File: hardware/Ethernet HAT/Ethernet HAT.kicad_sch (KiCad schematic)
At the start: 3 parts, among them J1 RJ45_Amphenol_RJMG1BD3B8K1ANR, J2 Conn_01x10_Pin, U1 W5500

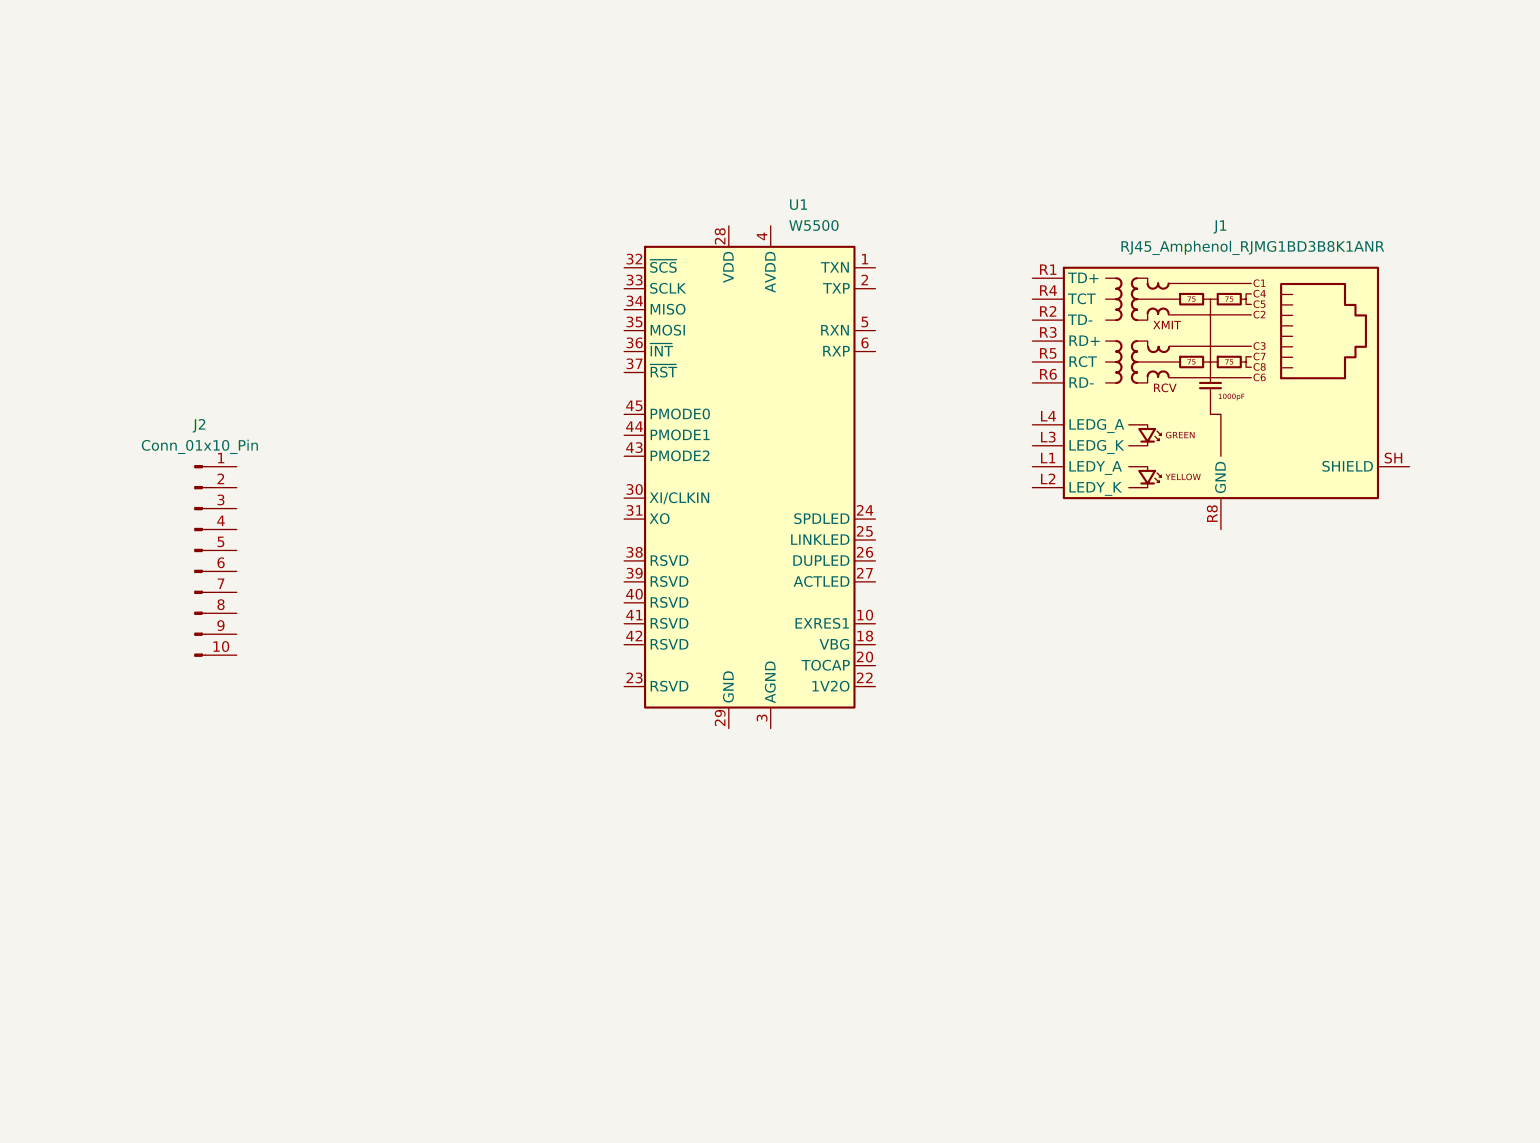
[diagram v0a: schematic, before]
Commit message: EthernetHat ordered
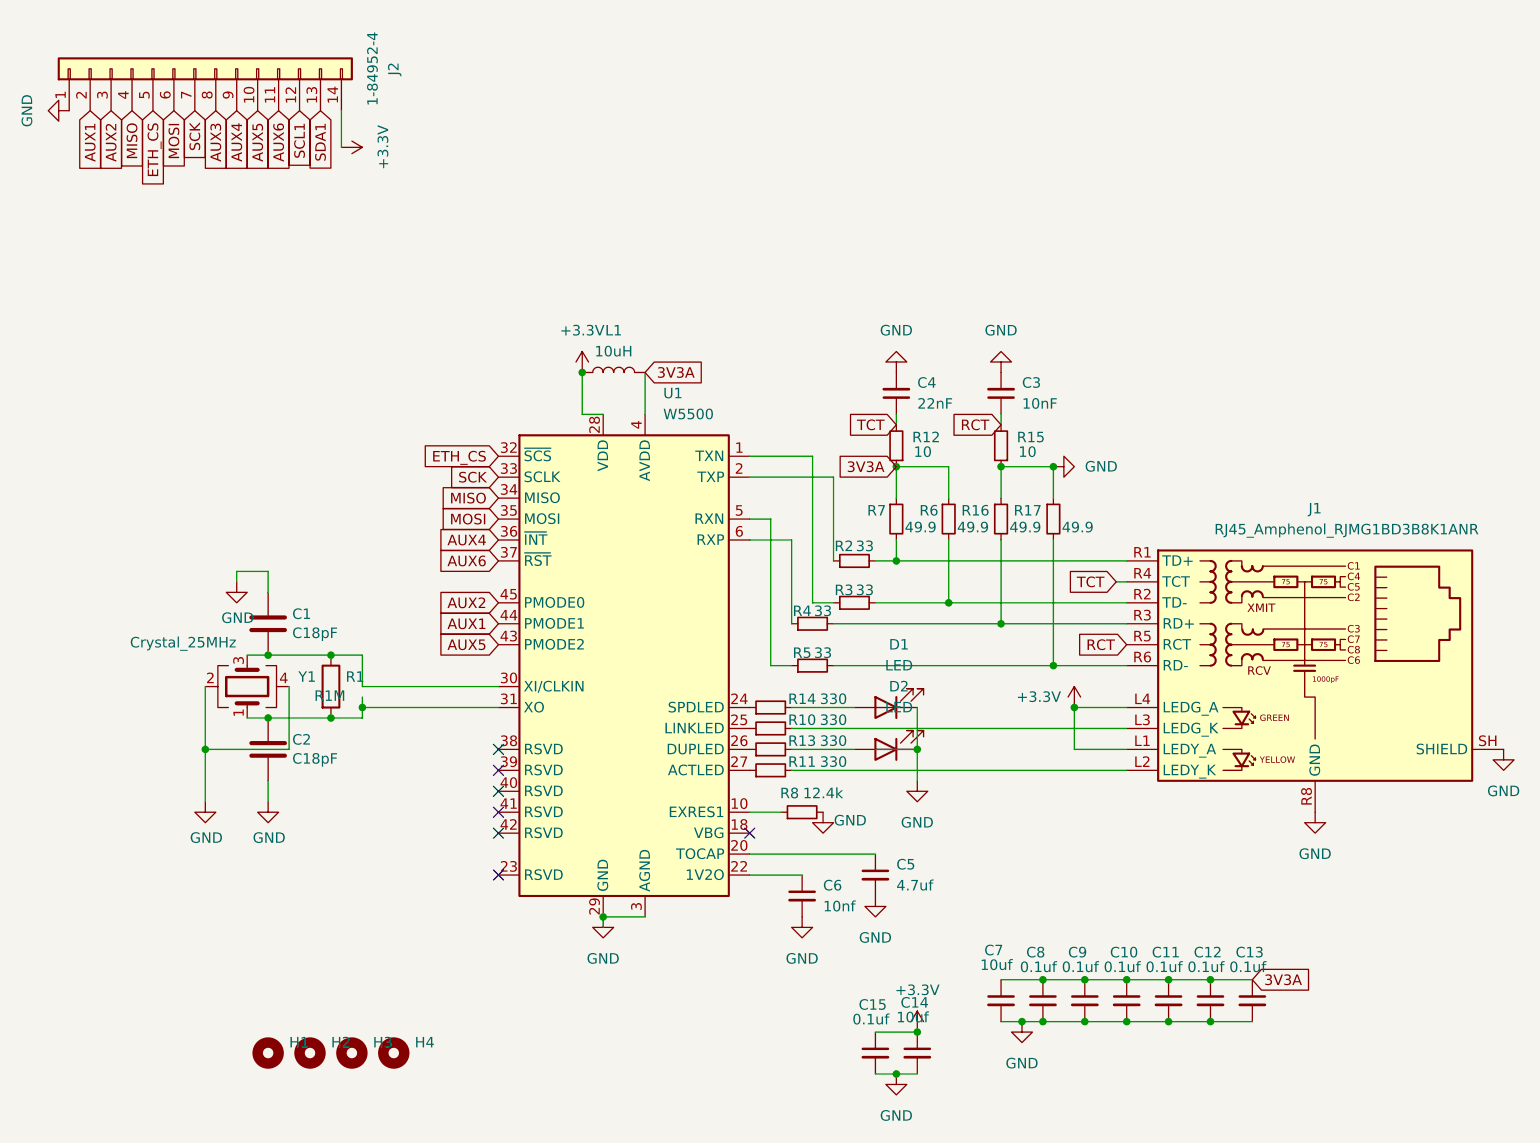
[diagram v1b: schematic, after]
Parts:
- removed J2: Conn_01x10_Pin, Connector_PinHeader_2.54mm:PinHeader_2x05_P2.54mm_Vertical, symbol Connector:Conn_01x10_Pin
- added C1, C2: C18pF, Capacitor_SMD:C_0402_1005Metric, symbol Device:C
- added C10, C11, C12, C13, C15, C8, C9: 0.1uf, Capacitor_SMD:C_0402_1005Metric, symbol Device:C_Small
- added C14, C7: 10uf, Capacitor_SMD:C_0805_2012Metric, symbol Device:C_Small
- added C3: 10nF, Capacitor_SMD:C_0402_1005Metric, symbol Device:C_Small
- added C4: 22nF, Capacitor_SMD:C_0402_1005Metric, symbol Device:C_Small
- added C5: 4.7uf, Capacitor_SMD:C_0402_1005Metric, symbol Device:C_Small
- added C6: 10nf, Capacitor_SMD:C_0402_1005Metric, symbol Device:C_Small
- added D1, D2: LED, LED_SMD:LED_0603_1608Metric, symbol Device:LED
- added H1, H2, H3, H4: MountingHole, MountingHole:MountingHole_3.2mm_M3_ISO14580_Pad, symbol Mechanical:MountingHole
- added J2: 1-84952-4, Connector_FFC-FPC:TE_1-84952-4_1x14-1MP_P1.0mm_Horizontal, symbol Connector_Generic:Conn_01x14
- added L1: 10uH, Inductor_SMD:L_0603_1608Metric, symbol Device:L
- added R1: R1M, Resistor_SMD:R_0402_1005Metric, symbol Device:R
- added R10, R11, R13, R14: 330, Resistor_SMD:R_0402_1005Metric, symbol Device:R_Small
- added R12, R15: 10, Resistor_SMD:R_0402_1005Metric, symbol Device:R_Small
- added R16, R17, R6, R7: 49.9, Resistor_SMD:R_0402_1005Metric, symbol Device:R_Small
- added R2, R3, R4, R5: 33, Resistor_SMD:R_0402_1005Metric, symbol Device:R_Small
- added R8: 12.4k, Resistor_SMD:R_0402_1005Metric, symbol Device:R_Small
- added Y1: Crystal_25MHz, Crystal:Crystal_SMD_3225-4Pin_3.2x2.5mm, symbol Device:Crystal_GND24
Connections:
- net +3.3V: now reaches J1.L1 (LEDY_A)
- net +3.3V: now also J1.L4 (LEDG_A), U1.28 (VDD), C14.1, C15.1, J2.14 (Pin_14), L1.1
- net at J1.L2 (LEDY_K): now also R11.2
- net at J1.L3 (LEDG_K): now also R10.2
- net at J1.R1 (TD+): now also R2.2, R7.2
- net at J1.R2 (TD-): now also R3.2, R6.2
- net at J1.R3 (RD+): now also R16.2, R4.2
- net TCT: now reaches J1.R4 (TCT)
- net TCT: now also C4.1, R12.2
- net RCT: now reaches J1.R5 (RCT)
- net RCT: now also C3.1, R15.2
- net at J1.R6 (RD-): now also R17.2, R5.2
- net GND: now reaches J1.R8 (GND)
- net GND: now also J1.SH (SHIELD), U1.14 (AGND), U1.16 (AGND), U1.19 (AGND), U1.29 (GND), U1.3 (AGND), U1.48 (AGND), U1.9 (AGND), C1.1, C10.2, C11.2, C12.2, C13.2, C14.2, C15.2, C2.2, C3.2, C4.2, C5.2, C6.2, C7.2, C8.2, C9.2, D1.1 (K), D2.1 (K), J2.1 (Pin_1), R15.1, R16.1, R17.1, R8.2, Y1.2, Y1.4
- net at U1.1 (TXN): now also R3.1
- net at U1.10 (EXRES1): now also R8.1
- net 3V3A: now reaches U1.11 (AVDD), U1.15 (AVDD), U1.17 (AVDD), U1.21 (AVDD), U1.4 (AVDD), U1.8 (AVDD)
- net 3V3A: now also C10.1, C11.1, C12.1, C13.1, C7.1, C8.1, C9.1, L1.2, R12.1, R6.1, R7.1
- net at U1.2 (TXP): now also R2.1
- net at U1.20 (TOCAP): now also C5.1
- net at U1.22 (1V2O): now also C6.1
- net at U1.24 (SPDLED): now also R14.1
- net at U1.25 (LINKLED): now also R10.1
- net at U1.26 (DUPLED): now also R13.1
- net at U1.27 (ACTLED): now also R11.1
- net at U1.30 (XI/CLKIN): now also C1.2, R1.1, Y1.3
- net at U1.31 (XO): now also C2.1, R1.2, Y1.1
- net ETH_CS: now reaches U1.32 (~{SCS})
- net ETH_CS: now also J2.5 (Pin_5)
- net SCK: now reaches U1.33 (SCLK)
- net SCK: now also J2.7 (Pin_7)
- net MISO: now reaches U1.34 (MISO)
- net MISO: now also J2.4 (Pin_4)
- net MOSI: now reaches U1.35 (MOSI)
- net MOSI: now also J2.6 (Pin_6)
- net AUX4: now reaches U1.36 (~{INT})
- net AUX4: now also J2.9 (Pin_9)
- net AUX6: now reaches U1.37 (~{RST})
- net AUX6: now also J2.11 (Pin_11)
- net AUX5: now reaches U1.43 (PMODE2)
- net AUX5: now also J2.10 (Pin_10)
- net AUX1: now reaches U1.44 (PMODE1)
- net AUX1: now also J2.2 (Pin_2)
- net AUX2: now reaches U1.45 (PMODE0)
- net AUX2: now also J2.3 (Pin_3)
- net at U1.5 (RXN): now also R5.1
- net at U1.6 (RXP): now also R4.1
- new net: D1.2 (A), R14.2
- new net: D2.2 (A), R13.2
- new net AUX3: J2.8 (Pin_8)
- new net SCL1: J2.12 (Pin_12)
- new net SDA1: J2.13 (Pin_13)
- no-connect marks 0 -> 7
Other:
- moved on the sheet: J1, U1
